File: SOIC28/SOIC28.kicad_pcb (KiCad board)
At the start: 2 copper layers, 35.8 x 18 mm, 7 parts, among them J1 Conn_01x14, J2 Conn_02x14_Counter_Clockwise, J3 Conn_01x14, J4 Conn_02x14_Counter_Clockwise

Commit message: Schematic PDF and 3D Renders added
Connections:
- J2 pad 8: Net-(J1-Pad8) -> Net-(J2-Pad28)
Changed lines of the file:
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@@
     (0 F.Cu signal)
     (31 B.Cu signal)
-    (32 B.Adhes user)
-    (33 F.Adhes user)
-    (34 B.Paste user)
-    (35 F.Paste user)
+    (32 B.Adhes user hide)
+    (33 F.Adhes user hide)
+    (34 B.Paste user hide)
+    (35 F.Paste user hide)
     (36 B.SilkS user)
     (37 F.SilkS user)
-    (38 B.Mask user)
-    (39 F.Mask user)
-    (40 Dwgs.User user)
+    (38 B.Mask user hide)
+    (39 F.Mask user hide)
+    (40 Dwgs.User user hide)
     (41 Cmts.User user hide)
     (42 Eco1.User user hide)
@@
     (mod_text_size 1 1)
     (mod_text_width 0.15)
-    (pad_size 1.7 1.7)
-    (pad_drill 1)
+    (pad_size 4.5 0.6)
+    (pad_drill 0)
     (pad_to_mask_clearance 0)
     (solder_mask_min_width 0.1)
@@
       (net 16 "Net-(J2-Pad27)"))
     (pad 8 smd roundrect (at 3.429 -8.255 270) (size 4.5 0.6) (layers F.Cu F.Paste F.Mask) (roundrect_rratio 0.25)
-      (net 7 "Net-(J1-Pad8)"))
+      (net 15 "Net-(J2-Pad28)"))
     (pad 21 smd roundrect (at 3.429 0.635 270) (size 4.5 0.6) (layers F.Cu F.Paste F.Mask) (roundrect_rratio 0.25)
       (net 22 "Net-(J2-Pad21)"))
@@
   (segment (start 62.4627 42.208) (end 61.1487 40.894) (width 0.2) (layer B.Cu) (net 14))
   (segment (start 61.1487 40.894) (end 55.499 40.894) (width 0.2) (layer B.Cu) (net 14))
-  (segment (start 58.42 33.808) (end 52.985 33.808) (width 0.2) (layer F.Cu) (net 15))
   (segment (start 52.985 33.808) (end 50.165 30.988) (width 0.2) (layer F.Cu) (net 15))
   (segment (start 61.2757 36.195) (end 62.4627 35.008) (width 0.2) (layer B.Cu) (net 15))
   (segment (start 50.1904 30.988) (end 55.3974 36.195) (width 0.2) (layer B.Cu) (net 15))
   (segment (start 55.3974 36.195) (end 61.2757 36.195) (width 0.2) (layer B.Cu) (net 15))
+  (segment (start 58.42 33.808) (end 52.985 33.808) (width 0.2) (layer F.Cu) (net 15))
   (via (at 55.372 34.925) (size 0.8) (drill 0.4) (layers F.Cu B.Cu) (net 16))
   (segment (start 63.1127 35.008) (end 63.1127 33.933) (width 0.2) (layer B.Cu) (net 16))

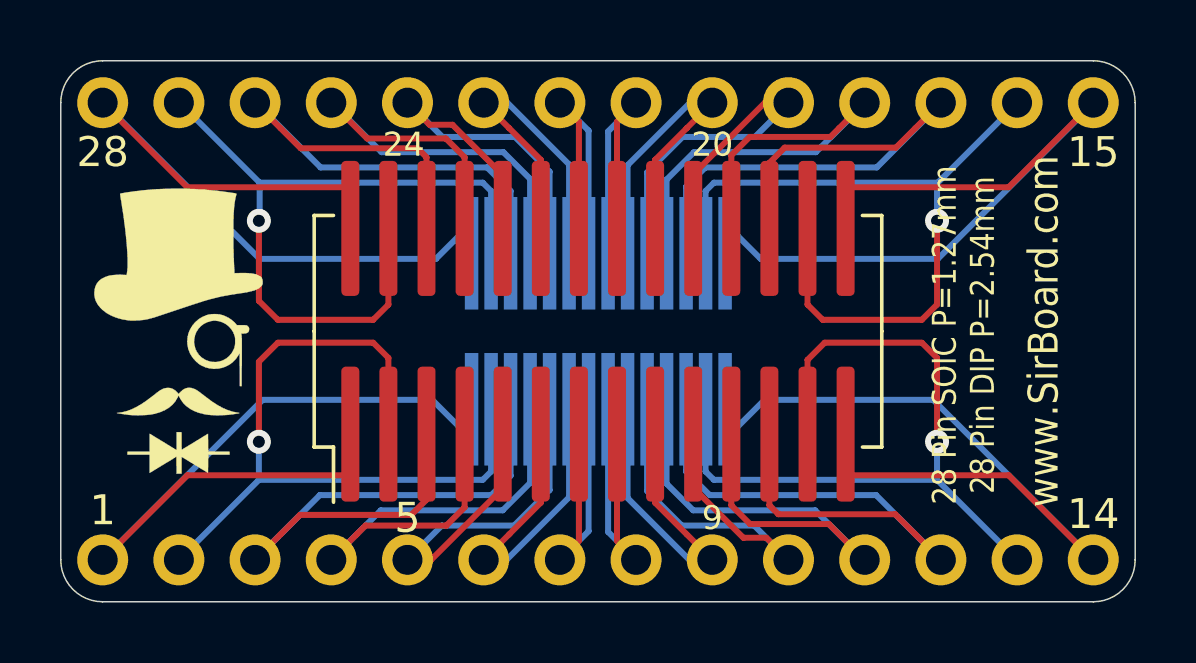
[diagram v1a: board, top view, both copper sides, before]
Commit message: Board Updates
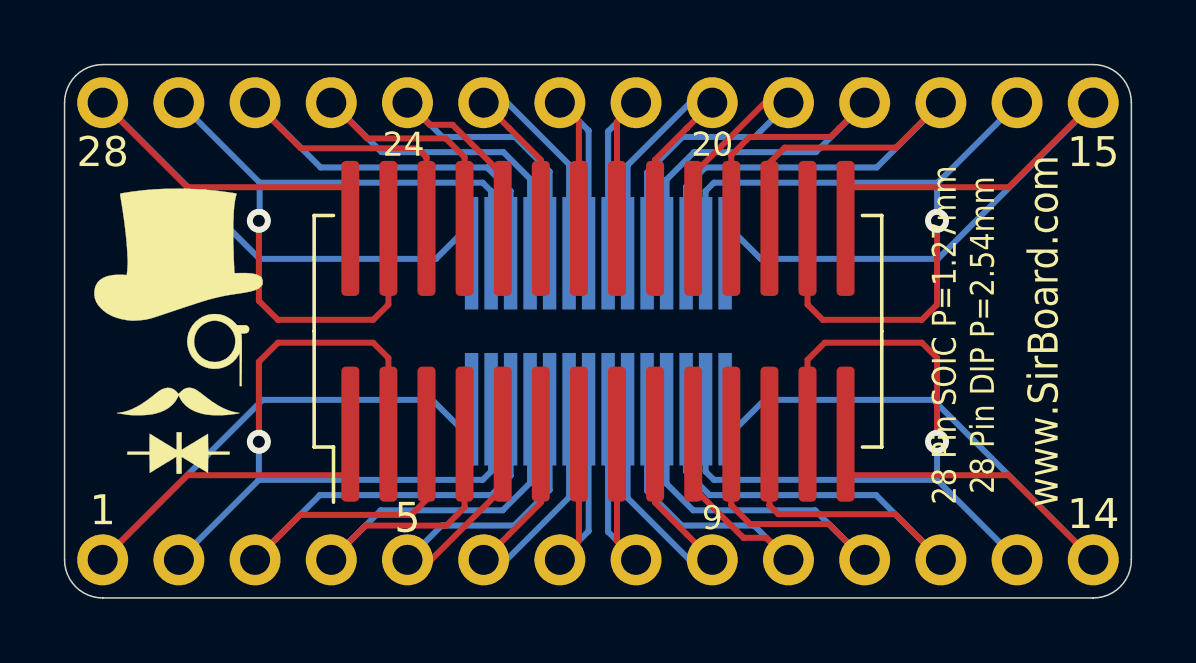
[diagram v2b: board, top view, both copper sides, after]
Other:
- board size 35.8 x 18 mm -> 35.6 x 17.8 mm
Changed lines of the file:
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@@
     (38 B.Mask user hide)
     (39 F.Mask user hide)
-    (40 Dwgs.User user hide)
+    (40 Dwgs.User user)
     (41 Cmts.User user hide)
     (42 Eco1.User user hide)
@@
       (xy -1.525562 0.880297)) (layer B.SilkS) (width 0.01))
   )
+  (gr_line (start 48.895 46.228) (end 48.895 30.988) (layer Edge.Cuts) (width 0.05))
+  (gr_line (start 83.185 47.498) (end 50.165 47.498) (layer Edge.Cuts) (width 0.05))
+  (gr_line (start 84.455 30.988) (end 84.455 46.228) (layer Edge.Cuts) (width 0.05))
+  (gr_line (start 50.165 29.718) (end 83.185 29.718) (layer Edge.Cuts) (width 0.05))
+  (gr_arc (start 83.185 30.988) (end 84.455 30.988) (angle -90) (layer Edge.Cuts) (width 0.05))
+  (gr_arc (start 83.185 46.228) (end 83.185 47.498) (angle -90) (layer Edge.Cuts) (width 0.05))
+  (gr_arc (start 50.165 46.228) (end 48.895 46.228) (angle -90) (layer Edge.Cuts) (width 0.05))
+  (gr_arc (start 50.165 30.988) (end 50.165 29.718) (angle -90) (layer Edge.Cuts) (width 0.05))
   (dimension 33.02 (width 0.15) (layer Dwgs.User)
     (gr_text "33.020 mm" (at 66.675 26.259) (layer Dwgs.User)
@@
     (arrow2b (pts (xy 50.165 27.559) (xy 51.291504 26.972579)))
   )
-  (dimension 35.814 (width 0.15) (layer Dwgs.User)
-    (gr_text "35.814 mm" (at 66.675 23.338) (layer Dwgs.User)
+  (dimension 35.56 (width 0.15) (layer Dwgs.User)
+    (gr_text "35.560 mm" (at 66.675 23.338) (layer Dwgs.User)
       (effects (font (size 1 1) (thickness 0.15)) hide)
     )
-    (feature1 (pts (xy 84.582 30.988) (xy 84.582 24.051579)))
-    (feature2 (pts (xy 48.768 30.988) (xy 48.768 24.051579)))
-    (crossbar (pts (xy 48.768 24.638) (xy 84.582 24.638)))
-    (arrow1a (pts (xy 84.582 24.638) (xy 83.455496 25.224421)))
-    (arrow1b (pts (xy 84.582 24.638) (xy 83.455496 24.051579)))
-    (arrow2a (pts (xy 48.768 24.638) (xy 49.894504 25.224421)))
-    (arrow2b (pts (xy 48.768 24.638) (xy 49.894504 24.051579)))
+    (feature1 (pts (xy 84.455 30.988) (xy 84.455 24.051579)))
+    (feature2 (pts (xy 48.895 30.988) (xy 48.895 24.051579)))
+    (crossbar (pts (xy 48.895 24.638) (xy 84.455 24.638)))
+    (arrow1a (pts (xy 84.455 24.638) (xy 83.328496 25.224421)))
+    (arrow1b (pts (xy 84.455 24.638) (xy 83.328496 24.051579)))
+    (arrow2a (pts (xy 48.895 24.638) (xy 50.021504 25.224421)))
+    (arrow2b (pts (xy 48.895 24.638) (xy 50.021504 24.051579)))
   )
   (dimension 15.24 (width 0.15) (layer Dwgs.User)
@@
     (arrow2b (pts (xy 46.863 46.228) (xy 46.276579 45.101496)))
   )
-  (dimension 18.034 (width 0.15) (layer Dwgs.User)
-    (gr_text "18.034 mm" (at 42.515 38.608 90) (layer Dwgs.User)
+  (dimension 17.78 (width 0.15) (layer Dwgs.User)
+    (gr_text "17.780 mm" (at 42.515 38.608 90) (layer Dwgs.User)
       (effects (font (size 1 1) (thickness 0.15)) hide)
     )
-    (feature1 (pts (xy 50.165 29.591) (xy 43.228579 29.591)))
-    (feature2 (pts (xy 50.165 47.625) (xy 43.228579 47.625)))
-    (crossbar (pts (xy 43.815 47.625) (xy 43.815 29.591)))
-    (arrow1a (pts (xy 43.815 29.591) (xy 44.401421 30.717504)))
-    (arrow1b (pts (xy 43.815 29.591) (xy 43.228579 30.717504)))
-    (arrow2a (pts (xy 43.815 47.625) (xy 44.401421 46.498496)))
-    (arrow2b (pts (xy 43.815 47.625) (xy 43.228579 46.498496)))
+    (feature1 (pts (xy 50.165 29.718) (xy 43.228579 29.718)))
+    (feature2 (pts (xy 50.165 47.498) (xy 43.228579 47.498)))
+    (crossbar (pts (xy 43.815 47.498) (xy 43.815 29.718)))
+    (arrow1a (pts (xy 43.815 29.718) (xy 44.401421 30.844504)))
+    (arrow1b (pts (xy 43.815 29.718) (xy 43.228579 30.844504)))
+    (arrow2a (pts (xy 43.815 47.498) (xy 44.401421 46.371496)))
+    (arrow2b (pts (xy 43.815 47.498) (xy 43.228579 46.371496)))
   )
   (gr_text 1 (at 50.165 44.577) (layer F.SilkS)
@@
     (effects (font (size 1 0.9) (thickness 0.15)))
   )
-  (gr_line (start 84.582 46.228) (end 84.582 30.988) (layer Edge.Cuts) (width 0.05))
-  (gr_line (start 50.165 47.625) (end 83.185 47.625) (layer Edge.Cuts) (width 0.05))
-  (gr_line (start 48.768 30.988) (end 48.768 46.228) (layer Edge.Cuts) (width 0.05))
-  (gr_line (start 83.185 29.591) (end 50.165 29.591) (layer Edge.Cuts) (width 0.05))
-  (gr_arc (start 83.185 30.988) (end 84.582 30.988) (angle -90) (layer Edge.Cuts) (width 0.05))
-  (gr_arc (start 83.185 46.228) (end 83.185 47.625) (angle -90) (layer Edge.Cuts) (width 0.05))
-  (gr_arc (start 50.165 46.228) (end 48.768 46.228) (angle -90) (layer Edge.Cuts) (width 0.05))
-  (gr_arc (start 50.165 30.988) (end 50.165 29.591) (angle -90) (layer Edge.Cuts) (width 0.05))
   (segment (start 80.365 43.408) (end 83.185 46.228) (width 0.2) (layer F.Cu) (net 1))
   (segment (start 74.93 43.408) (end 80.365 43.408) (width 0.2) (layer F.Cu) (net 1))
